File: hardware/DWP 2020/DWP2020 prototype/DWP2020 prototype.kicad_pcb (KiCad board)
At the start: 2 copper layers, 2 parts, among them U1 Teensy4.0, U2 SSD1351_128X128_LCD-bGeigieNa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

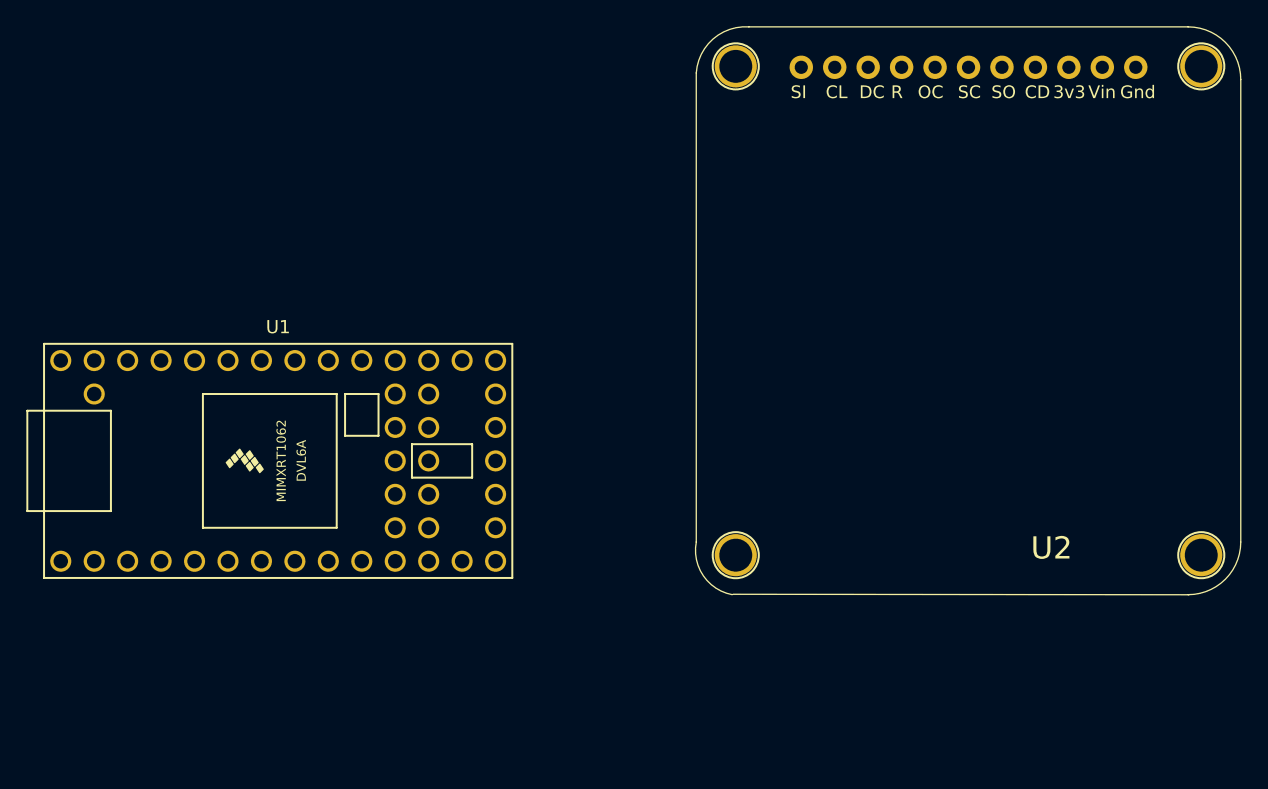
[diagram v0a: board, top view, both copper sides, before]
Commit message: fix some typoos
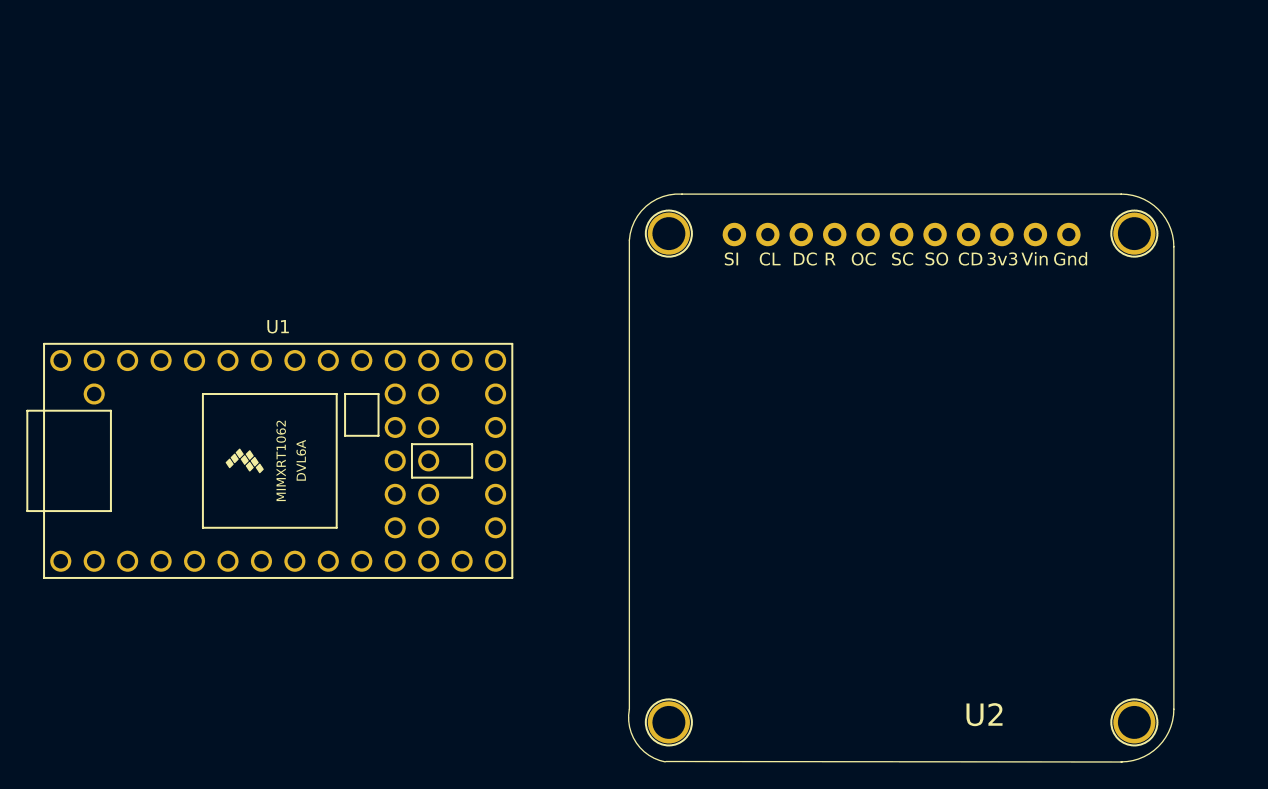
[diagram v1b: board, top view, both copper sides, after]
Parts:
- U2: value SSD1351_128X128_LCD-bGeigieNanoKit_V1.1r5a-eagle-import -> SSD1351_128X128
- moved U2 13.7 mm to (1008.4, 35.6)
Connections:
- U2 pad JP1$7: Net-(U2-PadJP1$7) -> Net-(U1-Pad33)
- U2 pad JP1$8: Net-(U2-PadJP1$8) -> Net-(U1-Pad1)
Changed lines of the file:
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@@
-(kicad_pcb (version 20200614) (host pcbnew "5.99.0-unknown-0bfe413~88~ubuntu18.04.1")
+(kicad_pcb (version 20200614) (host pcbnew "5.99.0-unknown-0dd34d1~88~ubuntu18.04.1")
   (general
     (thickness 1.6)
@@
     (tracks 0)
     (modules 2)
-    (nets 56)
+    (nets 54)
   )
   (paper "A4")
@@
   (net 49 "Net-(U2-PadJP1$5)")
   (net 50 "Net-(U2-PadJP1$6)")
-  (net 51 "Net-(U2-PadJP1$7)")
-  (net 52 "Net-(U2-PadJP1$8)")
-  (net 53 "Net-(U2-PadJP1$9)")
-  (net 54 "Net-(U2-PadJP1$10)")
-  (net 55 "Net-(U2-PadJP1$11)")
+  (net 51 "Net-(U2-PadJP1$9)")
+  (net 52 "Net-(U2-PadJP1$10)")
+  (net 53 "Net-(U2-PadJP1$11)")
   (net_class "Default" "This is the default net class."
     (clearance 0.2)
@@
     (add_net "Net-(U2-PadJP1$5)")
     (add_net "Net-(U2-PadJP1$6)")
-    (add_net "Net-(U2-PadJP1$7)")
-    (add_net "Net-(U2-PadJP1$8)")
     (add_net "Net-(U2-PadJP1$9)")
   )
   (module "DWP2020 prototype:SSD1351_128X128_LCD" (layer "F.Cu")
-    (at 1013.46 22.86)
+    (at 1008.38 35.56)
     (fp_text reference "U2" (at 6.35 20.32) (layer "F.SilkS")
       (effects (font (size 1.6891 1.6891) (thickness 0.135128)) (justify left bottom))
     )
-    (fp_text value "SSD1351_128X128_LCD-bGeigieNanoKit_V1.1r5a-eagle-import" (at 0 0) (layer "F.SilkS") hide
+    (fp_text value "SSD1351_128X128" (at 0 0) (layer "F.SilkS") hide
       (effects (font (size 1.27 1.27) (thickness 0.15)))
     )
@@
       (net 50 "Net-(U2-PadJP1$6)") (pinfunction "3.3V") (solder_mask_margin 0.1016))
     (pad "JP1$7" thru_hole circle (at 11.78499 -17.190009 90) (size 1.778 1.778) (drill 1) (layers *.Cu *.Mask)
-      (net 51 "Net-(U2-PadJP1$7)") (pinfunction "VDD") (solder_mask_margin 0.1016))
+      (net 25 "Net-(U1-Pad33)") (pinfunction "VDD") (solder_mask_margin 0.1016))
     (pad "JP1$8" thru_hole circle (at 14.32499 -17.190009 90) (size 1.778 1.778) (drill 1) (layers *.Cu *.Mask)
-      (net 52 "Net-(U2-PadJP1$8)") (pinfunction "GND") (solder_mask_margin 0.1016))
+      (net 11 "Net-(U1-Pad1)") (pinfunction "GND") (solder_mask_margin 0.1016))
     (pad "U$23$P$1" thru_hole circle (at 19.300012 -17.260012) (size 3.2 3.2) (drill 2.5) (layers *.Cu *.Mask)
       (solder_mask_margin 0.1016))
@@
       (solder_mask_margin 0.1016))
     (pad "JP1$9" thru_hole circle (at -11.075009 -17.190009 90) (size 1.778 1.778) (drill 1) (layers *.Cu *.Mask)
-      (net 53 "Net-(U2-PadJP1$9)") (pinfunction "SI") (solder_mask_margin 0.1016))
+      (net 51 "Net-(U2-PadJP1$9)") (pinfunction "SI") (solder_mask_margin 0.1016))
     (pad "JP1$10" thru_hole circle (at -8.535009 -17.190009 90) (size 1.778 1.778) (drill 1) (layers *.Cu *.Mask)
-      (net 54 "Net-(U2-PadJP1$10)") (pinfunction "CL") (solder_mask_margin 0.1016))
+      (net 52 "Net-(U2-PadJP1$10)") (pinfunction "CL") (solder_mask_margin 0.1016))
     (pad "JP1$11" thru_hole circle (at -5.995009 -17.190009 90) (size 1.778 1.778) (drill 1) (layers *.Cu *.Mask)
-      (net 55 "Net-(U2-PadJP1$11)") (pinfunction "DC") (solder_mask_margin 0.1016))
+      (net 53 "Net-(U2-PadJP1$11)") (pinfunction "DC") (solder_mask_margin 0.1016))
   )
   (module "Teensy:Teensy40" (layer "F.Cu")
